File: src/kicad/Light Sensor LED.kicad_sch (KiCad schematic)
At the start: 15 parts, among them J1 USB_A, U1 NE555P

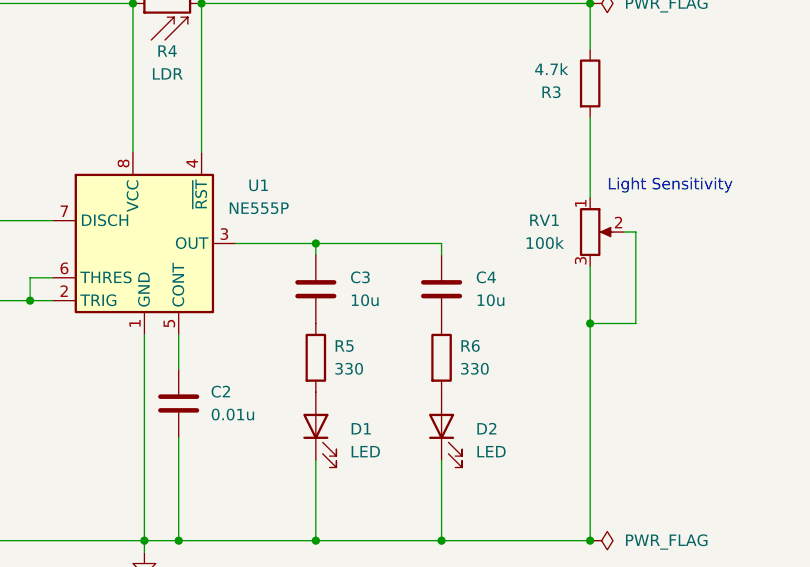
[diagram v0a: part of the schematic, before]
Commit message: Revised Project
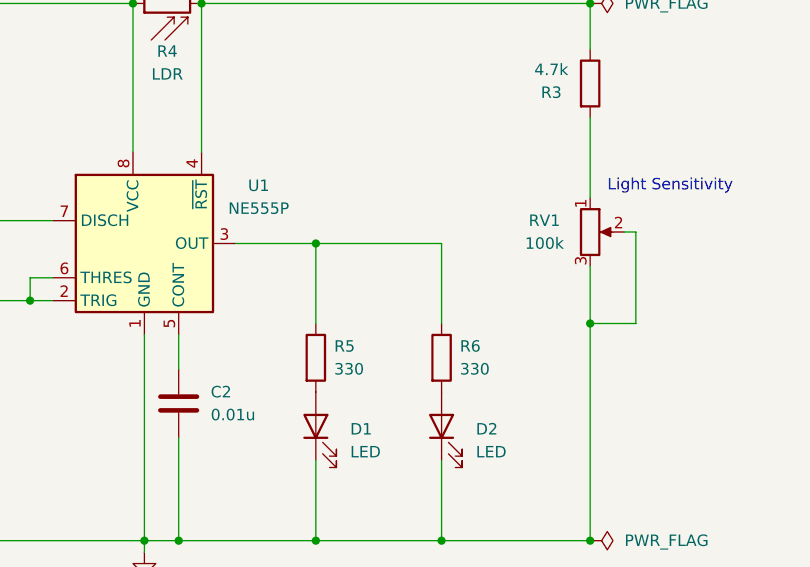
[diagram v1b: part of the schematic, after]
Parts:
- removed C3, C4: 10u, Capacitor_THT:C_Disc_D8.0mm_W5.0mm_P5.00mm, symbol Device:C
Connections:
- net at R6.1: now also R5.1, U1.3 (OUT)
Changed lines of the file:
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@@
-	(wire
-		(pts
-			(xy 156.21 87.63) (xy 156.21 88.9)
-		)
-		(stroke
-			(width 0)
-			(type default)
-		)
-	)
 	(wire
 		(pts
@@
 	(wire
 		(pts
+			(xy 170.18 87.63) (xy 170.18 96.52)
+		)
+		(stroke
+			(width 0)
+			(type default)
+		)
+	)
+	(wire
+		(pts
 			(xy 110.49 93.98) (xy 110.49 97.79)
 		)
@@
 	(wire
 		(pts
-			(xy 170.18 87.63) (xy 170.18 88.9)
-		)
-		(stroke
-			(width 0)
-			(type default)
-		)
-	)
-	(wire
-		(pts
 			(xy 140.97 109.22) (xy 140.97 120.65)
+		)
+		(stroke
+			(width 0)
+			(type default)
+		)
+	)
+	(wire
+		(pts
+			(xy 156.21 87.63) (xy 156.21 96.52)
 		)
 		(stroke
@@
 	)
 	(symbol
-		(lib_id "Device:C")
-		(at 156.21 92.71 0)
-		(unit 1)
-		(exclude_from_sim no)
-		(in_bom yes)
-		(on_board yes)
-		(dnp no)
-		(fields_autoplaced yes)
-		(property "Reference" "C3"
-			(at 160.02 91.4399 0)
-			(effects
-				(font
-					(size 1.27 1.27)
-				)
-				(justify left)
-			)
-		)
-		(property "Value" "10u"
-			(at 160.02 93.9799 0)
-			(effects
-				(font
-					(size 1.27 1.27)
-				)
-				(justify left)
-			)
-		)
-		(property "Footprint" "Capacitor_THT:C_Disc_D8.0mm_W5.0mm_P5.00mm"
-			(at 157.1752 96.52 0)
-			(effects
-				(font
-					(size 1.27 1.27)
-				)
-				(hide yes)
-			)
-		)
-		(property "Datasheet" "~"
-			(at 156.21 92.71 0)
-			(effects
-				(font
-					(size 1.27 1.27)
-				)
-				(hide yes)
-			)
-		)
-		(property "Description" "Unpolarized capacitor"
-			(at 156.21 92.71 0)
-			(effects
-				(font
-					(size 1.27 1.27)
-				)
-				(hide yes)
-			)
-		)
-		(pin "1"
-		)
-		(pin "2"
-		)
-		(instances
-			(project "Light Sensor LED"
-				(path "/200fe080-27c0-40e7-8309-972367add7fe"
-					(reference "C3")
-					(unit 1)
-				)
-			)
-		)
-	)
-	(symbol
 		(lib_id "Device:R")
 		(at 186.69 69.85 0)
@@
 					(unit 1)
 				)
-			)
-		)
-	)
-	(symbol
-		(lib_id "Device:C")
-		(at 170.18 92.71 0)
-		(unit 1)
-		(exclude_from_sim no)
-		(in_bom yes)
-		(on_board yes)
-		(dnp no)
-		(fields_autoplaced yes)
-		(property "Reference" "C4"
-			(at 173.99 91.4399 0)
-			(effects
-				(font
-					(size 1.27 1.27)
-				)
-				(justify left)
-			)
-		)
-		(property "Value" "10u"
-			(at 173.99 93.9799 0)
-			(effects
-				(font
-					(size 1.27 1.27)
-				)
-				(justify left)
-			)
-		)
-		(property "Footprint" "Capacitor_THT:C_Disc_D8.0mm_W5.0mm_P5.00mm"
-			(at 171.1452 96.52 0)
-			(effects
-				(font
-					(size 1.27 1.27)
-				)
-				(hide yes)
-			)
-		)
-		(property "Datasheet" "~"
-			(at 170.18 92.71 0)
-			(effects
-				(font
-					(size 1.27 1.27)
-				)
-				(hide yes)
-			)
-		)
-		(property "Description" "Unpolarized capacitor"
-			(at 170.18 92.71 0)
-			(effects
-				(font
-					(size 1.27 1.27)
-				)
-				(hide yes)
-			)
-		)
-		(pin "1"
-		)
-		(pin "2"
-		)
-		(instances
-			(project "Light Sensor LED"
-				(path "/200fe080-27c0-40e7-8309-972367add7fe"
-					(reference "C4")
-					(unit 1)
-				)
